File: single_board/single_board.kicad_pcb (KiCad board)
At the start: 4 copper layers, 100 x 100 mm, 126 parts, among them J11 SPI Debug, J17 BOOTSEL, J2 USB_C_Receptacle_USB2.0_16P, J3 SWD, J30 JST_GH_H, J31 JST_GH_H, J33 JST_GH_H, J34 PB_Vertical, J35 JST_GH_H, J36 JST_GH_H, J37 JST_GH_H, J38 PB_Vertical, J39 PB_Vertical, J40 PB_Vertical, J41 PB_Vertical, J42 PB_Vertical, J43 PB_Vertical, J44 PB_Vertical, J45 PB_Vertical, J46 PB_Vertical, J47 PB_Vertical, J48 PB_Vertical, J49 PB_Vertical, J5 JST-GH, J50 PB_Vertical, J53 PB_Vertical, J55 PB_Vertical, J56 Power, J57 PB_Vertical, J6 JST-GH, Q1 AO3400A, Q3 AO3401A, SW1 Button, U1 AP2112K-3.3, U3 USBLC6-2SC6, U4 LSM6DSV, U5 STM32G474VBTx, Y2 ABM8-16MHz

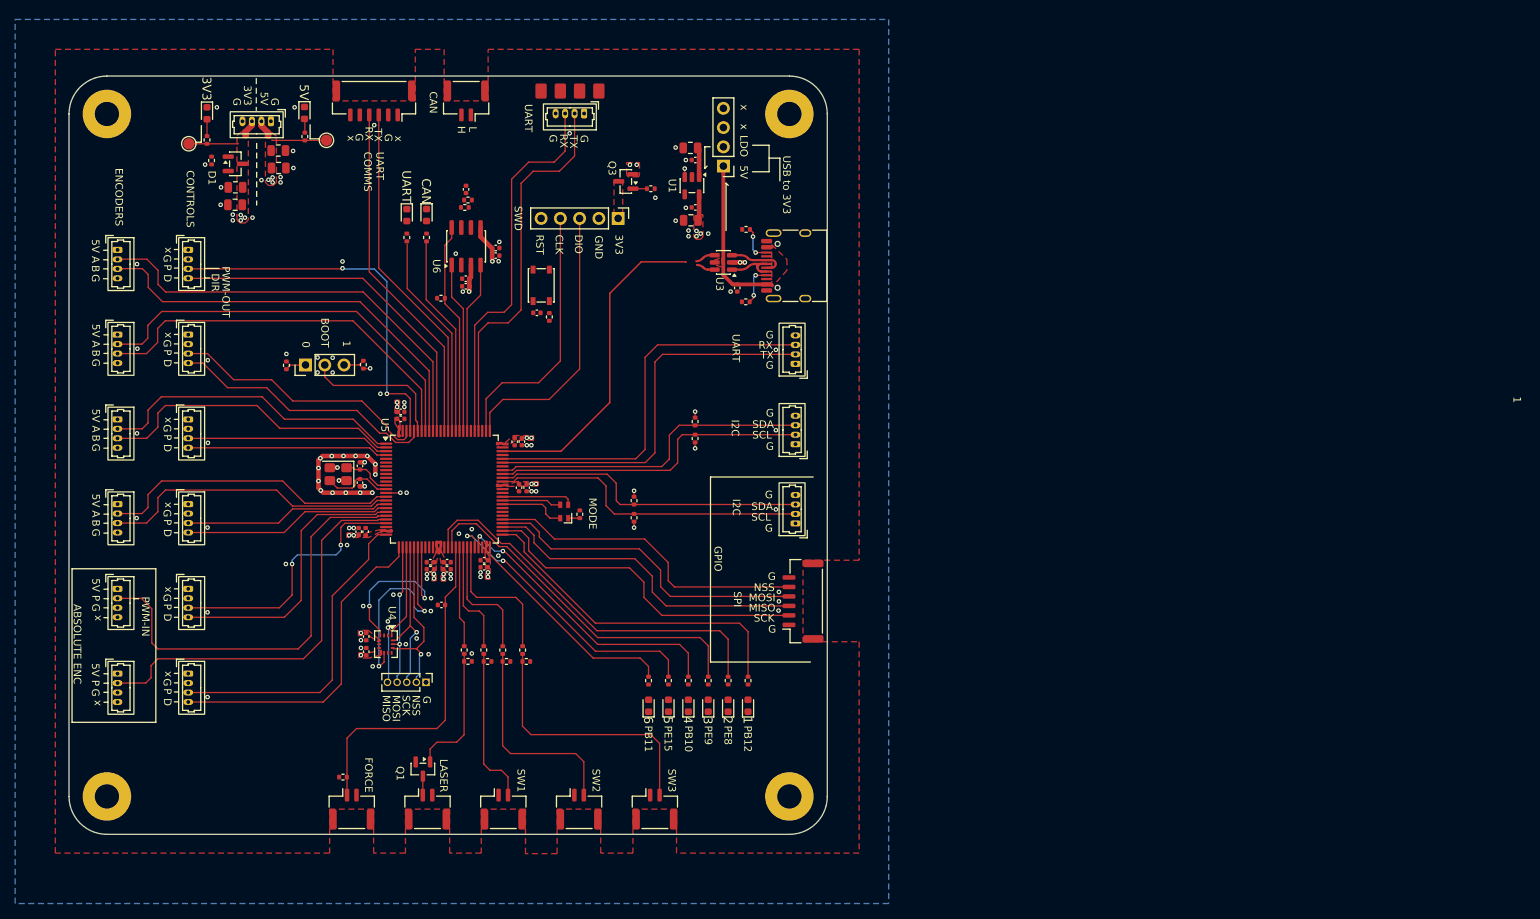
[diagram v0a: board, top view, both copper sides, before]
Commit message: CAN Diff Pair
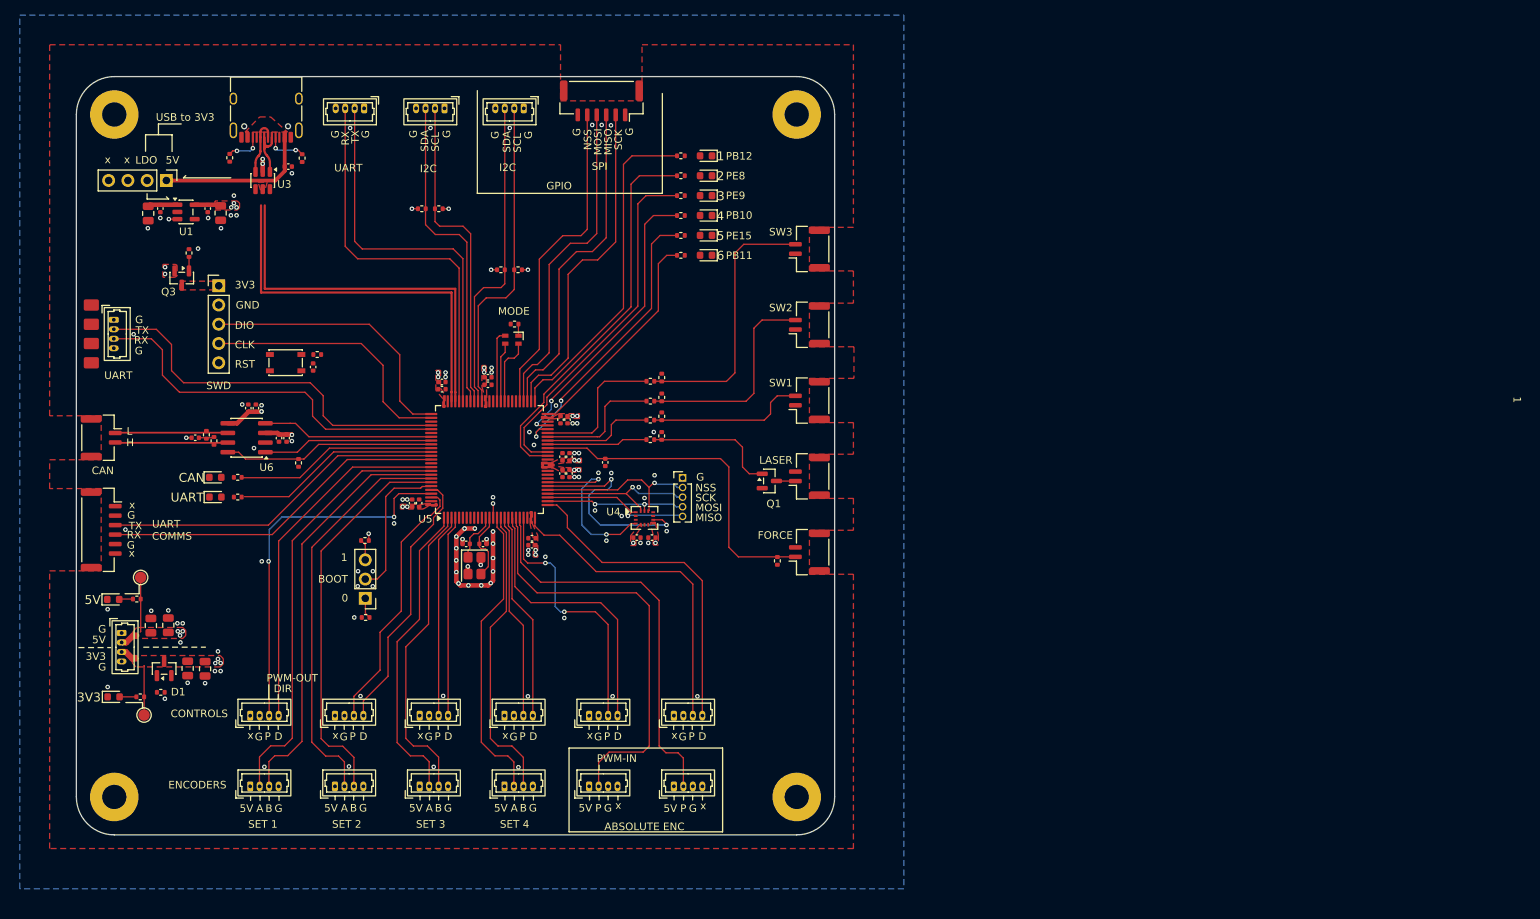
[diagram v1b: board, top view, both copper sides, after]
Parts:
- moved H2 91.0 mm to (143.3, 121.4), turned to 90 degrees
- moved H1 90.1 mm to (53.4, 121.4), turned to 90 degrees
- moved H4 89.9 mm to (143.3, 31.4), turned to 90 degrees
- moved H3 89.0 mm to (53.4, 31.4), turned to 90 degrees
- moved D4 77.9 mm to (53.3, 108.2), turned to 0 degrees
- moved J33 76.6 mm to (145.0, 49.2), turned to 90 degrees
- moved TP2 75.6 mm to (57.3, 110.6), turned to 0 degrees
- moved J43 74.9 mm to (127.2, 120.0), turned to 0 degrees
- moved R15 74.0 mm to (56.8, 108.2), turned to 180 degrees
- moved J56 73.5 mm to (60.2, 40.1), turned to -90 degrees
- moved J2 73.1 mm to (73.4, 30.4), turned to 180 degrees
- moved J39 72.9 mm to (71.3, 120.0), turned to 0 degrees
- moved D8 72.7 mm to (131.4, 36.9), turned to 180 degrees
- moved J54 72.0 mm to (48.3, 64.2), turned to 90 degrees
- moved C31 72.0 mm to (57.8, 44.5), turned to -90 degrees
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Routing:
- net /USB-DN: track 2.51 -> 51.0 mm
- net /CAN_DP: track 0.00 -> 14.9 mm
- net /CAN_DN: track 0.00 -> 14.9 mm
- net /USB-DP: track 45.7 -> 51.0 mm
- net Net-(C41-Pad1): track 0.00 -> 2.05 mm
- net GND: track 25.6 -> 26.3 mm, vias 102 -> 103
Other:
- board text added: "Absolute encoder position for lower Arm motors"
- board text added: "Drivebase Motors use standard CAN frames"
- board text added: "FDCAN"
- board text added: "Quadrature encoder input A/B : Ch1/Ch2 Reconfig Absolute encoder position PWM Input on Ch1 or Ch2"
- board text added: "SET 1"
- board text added: "SET 2"
- board text added: "SET 3"
- board text added: "SET 4"
- board text removed: "FDCAN/CAN"
